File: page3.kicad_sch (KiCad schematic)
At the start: 23 parts, among them Q1 MMBT3904-7-F, U16 40106, U18 TL082, U19 CD4094

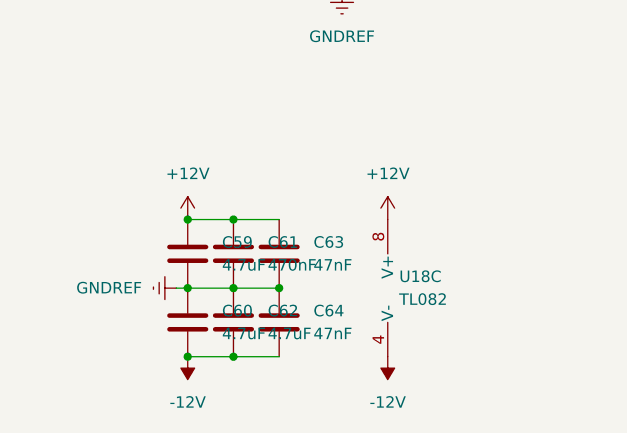
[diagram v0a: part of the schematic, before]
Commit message: routed 100%
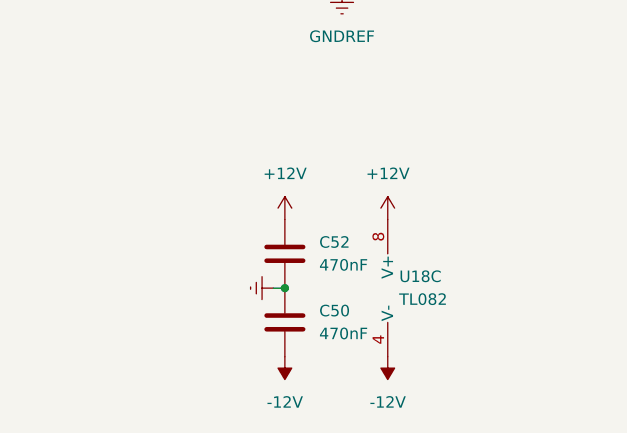
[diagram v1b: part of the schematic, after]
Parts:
- removed C59, C60, C62: 4.7uF, Capacitor_SMD:C_0805_2012Metric, symbol Device:C
- removed C61: 470nF, Capacitor_SMD:C_0805_2012Metric, symbol Device:C
- removed C63, C64: 47nF, Capacitor_SMD:C_0603_1608Metric, symbol Device:C
- added C50, C52: 470nF, Capacitor_SMD:C_0805_2012Metric, symbol Device:C
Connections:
- net +12V: now also C52.1
- net -12V: now also C50.2
- net GNDREF: now also C50.1, C52.2
